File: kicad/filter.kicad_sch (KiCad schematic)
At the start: 31 parts, among them J4 Conn_01x05, U4 NE5532, U5 NE5532, U6 NE5532, U7 NE5532

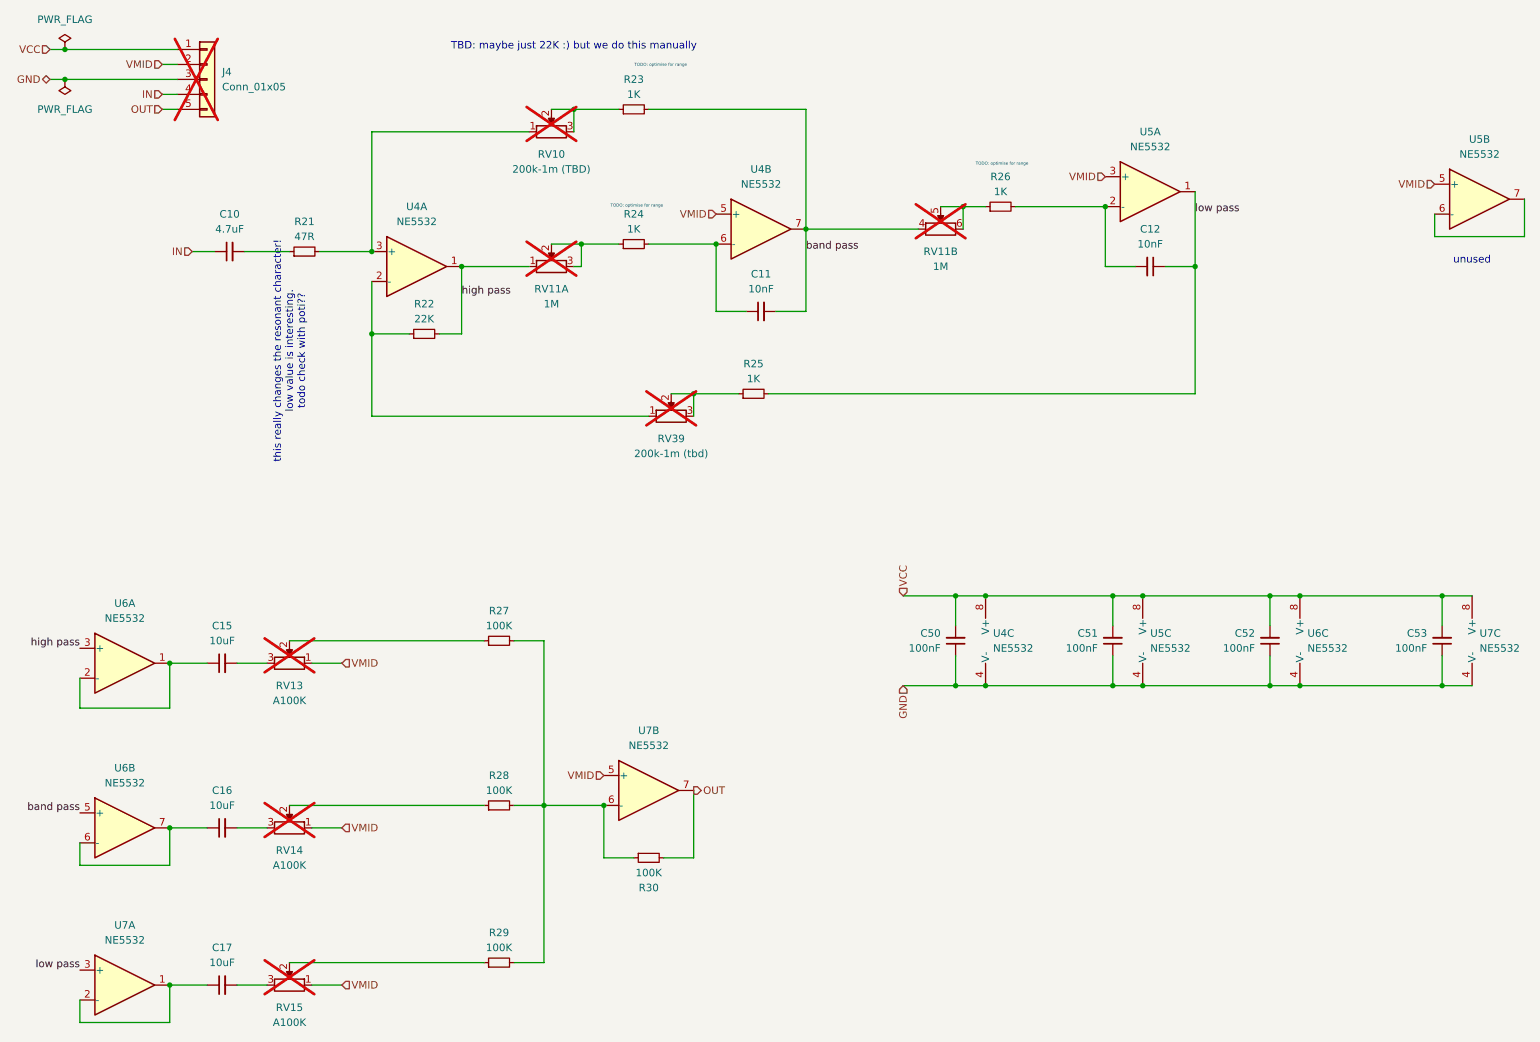
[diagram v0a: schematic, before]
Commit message: add local changes
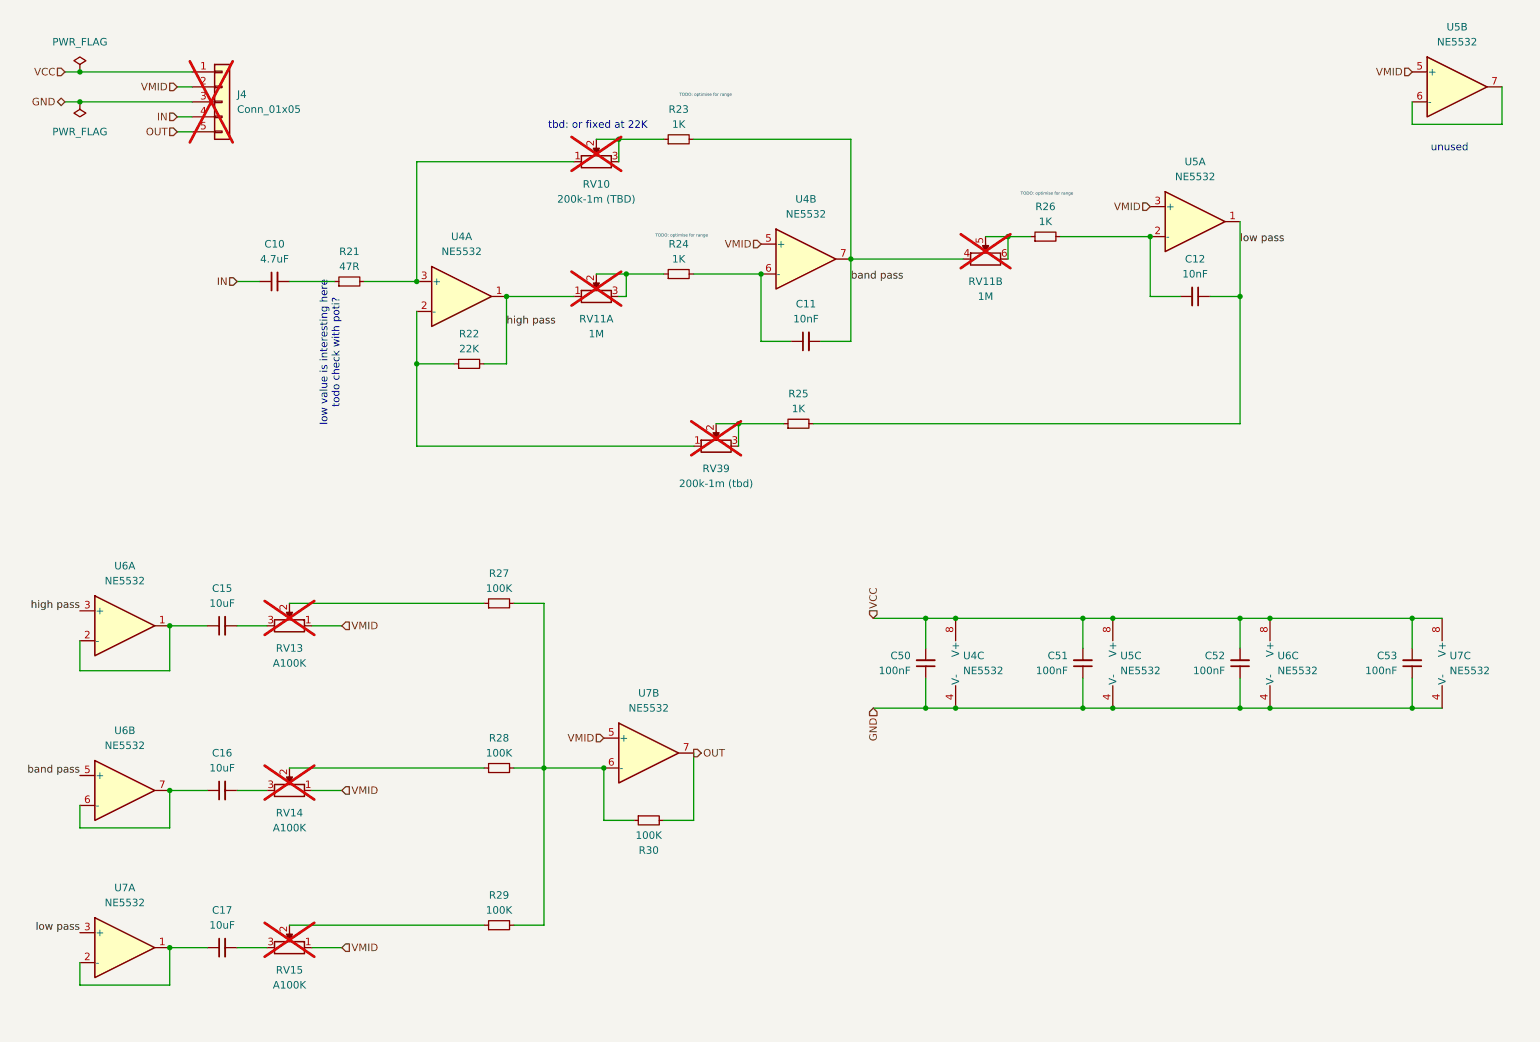
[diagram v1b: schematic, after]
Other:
- note added: "low value is interesting here todo check with poti?"
- note added: "tbd: or fixed at 22K"
- note removed: "TBD: maybe just 22K :) but we do this manually"
- note removed: "this really changes the resonant character! low value is interesting. todo check with poti??"
- moved on the sheet: C10, C11, C12, C15, C16, C17, C50, C51, C52, C53, J4, R21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
